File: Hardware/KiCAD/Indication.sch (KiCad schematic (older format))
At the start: 26 parts, among them Q1 2N7002, Q2 2N7002, Q3 2N7002, Q4 2N7002, Q5 2N7002

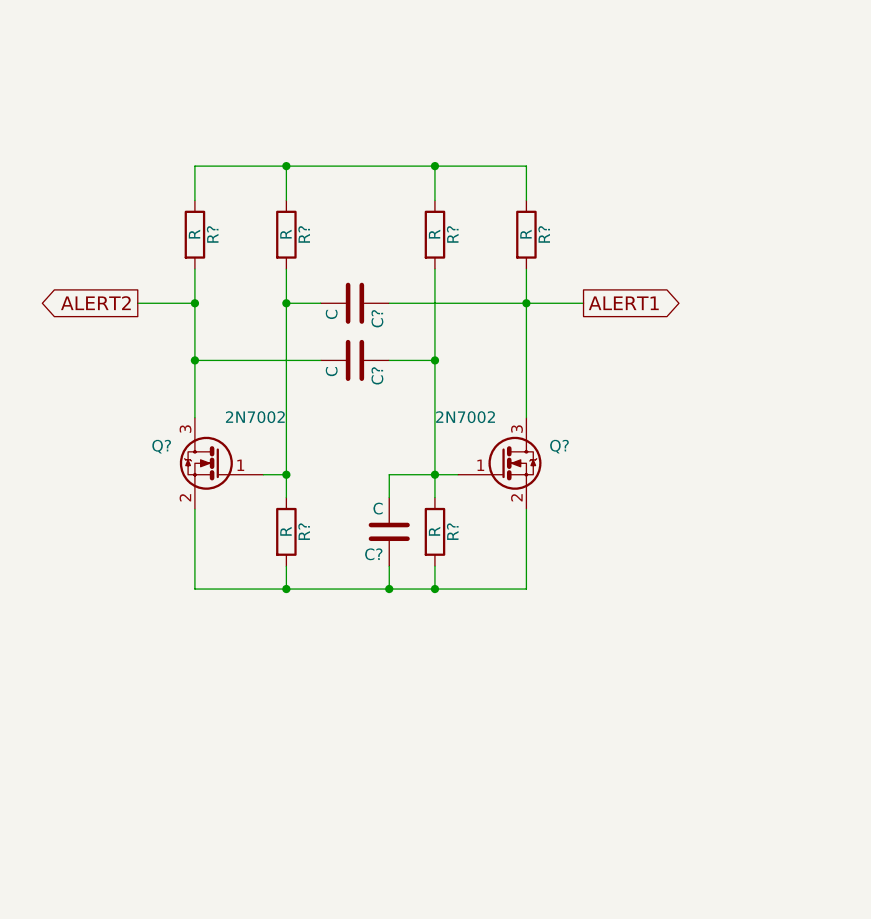
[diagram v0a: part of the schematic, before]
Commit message: more work on the schematic
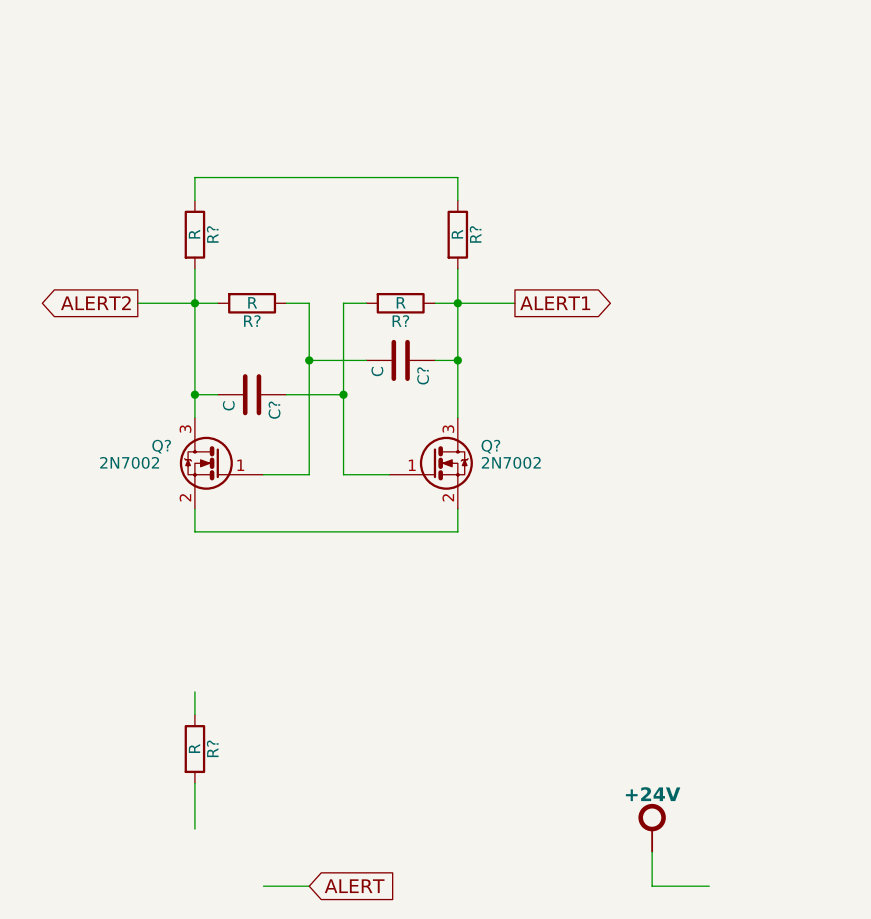
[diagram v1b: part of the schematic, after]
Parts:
- removed C?: C, symbol C
- removed R? (x2): R, symbol R
- added R?: R, symbol R
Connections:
- net labels added: +24V_BJH, ALERT
- wire segments 48 -> 50
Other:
- moved on the sheet: C?, Q?, R?
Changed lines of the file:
@@
 LIBS:Relays
 LIBS:Transistors-BJH
+LIBS:MemoryDevices-BJH
 LIBS:ptws-cache
 EELAYER 25 0
@@
 L 2N7002 Q?
 U 1 1 5806E246
-P 2600 4650
-F 0 "Q?" H 2800 4725 50  0000 L CNN
-F 1 "2N7002" H 2300 4850 50  0000 L CNN
-F 2 "" H 2800 4575 50  0000 L CIN
-F 3 "" H 2600 4650 50  0000 L CNN
-	1    2600 4650
+P 2300 4650
+F 0 "Q?" H 2500 4725 50  0000 L CNN
+F 1 "2N7002" H 2500 4650 50  0000 L CNN
+F 2 "" H 2500 4575 50  0000 L CIN
+F 3 "" H 2300 4650 50  0000 L CNN
+	1    2300 4650
 	1    0    0    -1
 $EndComp
@@
 P 1350 4650
 F 0 "Q?" H 1550 4725 50  0000 L CNN
-F 1 "2N7002" H 1050 4850 50  0000 L CNN
+F 1 "2N7002" H 1600 4650 50  0000 L CNN
 F 2 "" H 1550 4575 50  0000 L CIN
 F 3 "" H 1350 4650 50  0000 L CNN
@@
 L R R?
 U 1 1 5806E7DC
-P 1650 3650
-F 0 "R?" V 1730 3650 50  0000 C CNN
-F 1 "R" V 1650 3650 50  0000 C CNN
-F 2 "" V 1580 3650 50  0000 C CNN
-F 3 "" H 1650 3650 50  0000 C CNN
-	1    1650 3650
-	1    0    0    -1
+P 1500 3950
+F 0 "R?" V 1580 3950 50  0000 C CNN
+F 1 "R" V 1500 3950 50  0000 C CNN
+F 2 "" V 1430 3950 50  0000 C CNN
+F 3 "" H 1500 3950 50  0000 C CNN
+	1    1500 3950
+	0    1    1    0
 $EndComp
 $Comp
 L C C?
 U 1 1 5806E856
-P 1950 3950
-F 0 "C?" H 1975 4050 50  0000 L CNN
-F 1 "C" H 1975 3850 50  0000 L CNN
-F 2 "" H 1988 3800 50  0000 C CNN
-F 3 "" H 1950 3950 50  0000 C CNN
-	1    1950 3950
+P 1500 4350
+F 0 "C?" H 1525 4450 50  0000 L CNN
+F 1 "C" H 1525 4250 50  0000 L CNN
+F 2 "" H 1538 4200 50  0000 C CNN
+F 3 "" H 1500 4350 50  0000 C CNN
+	1    1500 4350
 	0    1    1    0
 $EndComp
@@
 L R R?
 U 1 1 5806E913
-P 2700 3650
-F 0 "R?" V 2780 3650 50  0000 C CNN
-F 1 "R" V 2700 3650 50  0000 C CNN
-F 2 "" V 2630 3650 50  0000 C CNN
-F 3 "" H 2700 3650 50  0000 C CNN
-	1    2700 3650
+P 2400 3650
+F 0 "R?" V 2480 3650 50  0000 C CNN
+F 1 "R" V 2400 3650 50  0000 C CNN
+F 2 "" V 2330 3650 50  0000 C CNN
+F 3 "" H 2400 3650 50  0000 C CNN
+	1    2400 3650
 	1    0    0    -1
 $EndComp
@@
 L R R?
 U 1 1 5806E9B1
-P 2300 3650
-F 0 "R?" V 2380 3650 50  0000 C CNN
-F 1 "R" V 2300 3650 50  0000 C CNN
-F 2 "" V 2230 3650 50  0000 C CNN
-F 3 "" H 2300 3650 50  0000 C CNN
-	1    2300 3650
-	1    0    0    -1
+P 2150 3950
+F 0 "R?" V 2230 3950 50  0000 C CNN
+F 1 "R" V 2150 3950 50  0000 C CNN
+F 2 "" V 2080 3950 50  0000 C CNN
+F 3 "" H 2150 3950 50  0000 C CNN
+	1    2150 3950
+	0    1    1    0
 $EndComp
 $Comp
 L C C?
 U 1 1 5806EB77
-P 1950 4200
-F 0 "C?" H 1975 4300 50  0000 L CNN
-F 1 "C" H 1975 4100 50  0000 L CNN
-F 2 "" H 1988 4050 50  0000 C CNN
-F 3 "" H 1950 4200 50  0000 C CNN
-	1    1950 4200
+P 2150 4200
+F 0 "C?" H 2175 4300 50  0000 L CNN
+F 1 "C" H 2175 4100 50  0000 L CNN
+F 2 "" H 2188 4050 50  0000 C CNN
+F 3 "" H 2150 4200 50  0000 C CNN
+	1    2150 4200
 	0    1    1    0
 $EndComp
-$Comp
-L R R?
-U 1 1 5806F01F
-P 1650 4950
-F 0 "R?" V 1730 4950 50  0000 C CNN
-F 1 "R" V 1650 4950 50  0000 C CNN
-F 2 "" V 1580 4950 50  0000 C CNN
-F 3 "" H 1650 4950 50  0000 C CNN
-	1    1650 4950
-	1    0    0    -1
-$EndComp
-$Comp
-L R R?
-U 1 1 5806F0AD
-P 2300 4950
-F 0 "R?" V 2380 4950 50  0000 C CNN
-F 1 "R" V 2300 4950 50  0000 C CNN
-F 2 "" V 2230 4950 50  0000 C CNN
-F 3 "" H 2300 4950 50  0000 C CNN
-	1    2300 4950
-	1    0    0    -1
-$EndComp
-$Comp
-L C C?
-U 1 1 5806F2D0
-P 2100 4950
-F 0 "C?" H 2125 5050 50  0000 L CNN
-F 1 "C" H 2125 4850 50  0000 L CNN
-F 2 "" H 2138 4800 50  0000 C CNN
-F 3 "" H 2100 4950 50  0000 C CNN
-	1    2100 4950
-	-1   0    0    1
-$EndComp
-Text GLabel 2950 3950 2    60   Output ~ 0
+Text GLabel 2650 3950 2    60   Output ~ 0
 ALERT1
 Wire Wire Line
@@
 	1250 3800 1250 4450
 Wire Wire Line
-	2700 3800 2700 4450
-Wire Wire Line
-	2300 3800 2300 4800
-Wire Wire Line
-	2100 4700 2400 4700
-Wire Wire Line
-	1650 3800 1650 4800
-Wire Wire Line
-	1650 4700 1550 4700
-Wire Wire Line
-	1800 3950 1650 3950
-Connection ~ 1650 3950
-Wire Wire Line
-	2100 3950 2950 3950
-Connection ~ 2700 3950
-Wire Wire Line
-	2100 4200 2300 4200
-Connection ~ 2300 4200
-Wire Wire Line
-	1800 4200 1250 4200
-Connection ~ 1250 4200
-Wire Wire Line
-	1250 3350 1250 3500
-Wire Wire Line
-	1250 3350 2700 3350
-Wire Wire Line
-	2700 3350 2700 3500
-Wire Wire Line
-	2300 3500 2300 3350
-Connection ~ 2300 3350
-Wire Wire Line
-	1650 3500 1650 3350
-Connection ~ 1650 3350
-Connection ~ 1650 4700
-Connection ~ 2300 4700
-Wire Wire Line
-	2100 4800 2100 4700
-Wire Wire Line
-	2700 4850 2700 5200
-Wire Wire Line
-	2700 5200 1250 5200
-Wire Wire Line
-	1250 5200 1250 4850
-Wire Wire Line
-	1650 5100 1650 5200
-Connection ~ 1650 5200
-Wire Wire Line
-	2100 5100 2100 5200
-Connection ~ 2100 5200
-Wire Wire Line
-	2300 5100 2300 5200
-Connection ~ 2300 5200
+	2400 3800 2400 4450
+Wire Wire Line
+	1750 4700 1550 4700
+Connection ~ 2400 3950
+Wire Wire Line
+	1250 3400 1250 3500
+Wire Wire Line
+	2400 3400 2400 3500
 Text GLabel 1000 3950 0    60   Output ~ 0
 ALERT2
 Wire Wire Line
-	1000 3950 1250 3950
+	1000 3950 1350 3950
 Connection ~ 1250 3950
+Wire Wire Line
+	2300 3950 2650 3950
+Wire Wire Line
+	1650 3950 1750 3950
+Wire Wire Line
+	1750 3950 1750 4700
+Wire Wire Line
+	2300 4200 2400 4200
+Connection ~ 2400 4200
+Wire Wire Line
+	2000 3950 1900 3950
+Wire Wire Line
+	1900 3950 1900 4700
+Wire Wire Line
+	1900 4700 2100 4700
+Wire Wire Line
+	1350 4350 1250 4350
+Connection ~ 1250 4350
+Wire Wire Line
+	1650 4350 1900 4350
+Connection ~ 1900 4350
+Wire Wire Line
+	2000 4200 1750 4200
+Connection ~ 1750 4200
+Wire Wire Line
+	2400 4850 2400 4950
+Wire Wire Line
+	2400 4950 1250 4950
+Wire Wire Line
+	1250 4950 1250 4850
+Wire Wire Line
+	1250 3400 2400 3400
+Text GLabel 1750 6500 2    60   Input ~ 0
+ALERT
+$Comp
+L +24V_BJH #PWR?
+U 1 1 58161080
+P 3250 6300
+F 0 "#PWR?" H 3250 6490 20  0001 C CNN
+F 1 "+24V_BJH" H 3250 6490 51  0001 C CNN
+F 2 "" H 3250 6300 60  0001 C CNN
+F 3 "" H 3250 6300 60  0001 C CNN
+F 4 "+24V" H 3250 6500 60  0000 C CNB "NAME"
+	1    3250 6300
+	1    0    0    -1
+$EndComp
+$Comp
+L R R?
+U 1 1 581610E5
+P 1250 5900
+F 0 "R?" V 1330 5900 50  0000 C CNN
+F 1 "R" V 1250 5900 50  0000 C CNN
+F 2 "" V 1180 5900 50  0000 C CNN
+F 3 "" H 1250 5900 50  0000 C CNN
+	1    1250 5900
+	1    0    0    -1
+$EndComp
+Wire Wire Line
+	1250 5650 1250 5750
+Wire Wire Line
+	1250 6050 1250 6250
+Wire Wire Line
+	1750 6500 1550 6500
+Wire Wire Line
+	3250 6350 3250 6500
+Wire Wire Line
+	3250 6500 3500 6500
 $EndSCHEMATC
